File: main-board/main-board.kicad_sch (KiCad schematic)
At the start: 89 parts, among them IC13 TPS2121RUXR, J47 Barrel Jack, J6 Conn_01x03, J66 Conn_01x01_Socket, J7 Conn_Boaxial, J73 Conn_01x03, J8 USB_C_Receptacle_USB2.0_16P, J9 Conn_02x04_Odd_Even, SW1 SW_Push, SW5 SW_Push, U10 SI5351A-B-GTR, U3 TLV75801PDBV, U5 TLV75801PDBV, X1 OK322532.768KJBA4SL, Y2 NX3225GA-25.000M-STD-CRG-2

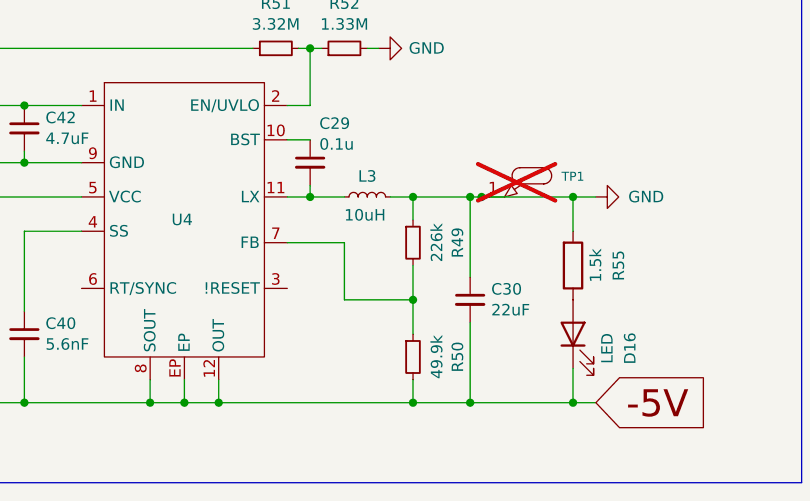
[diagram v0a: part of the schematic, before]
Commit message: pcb update
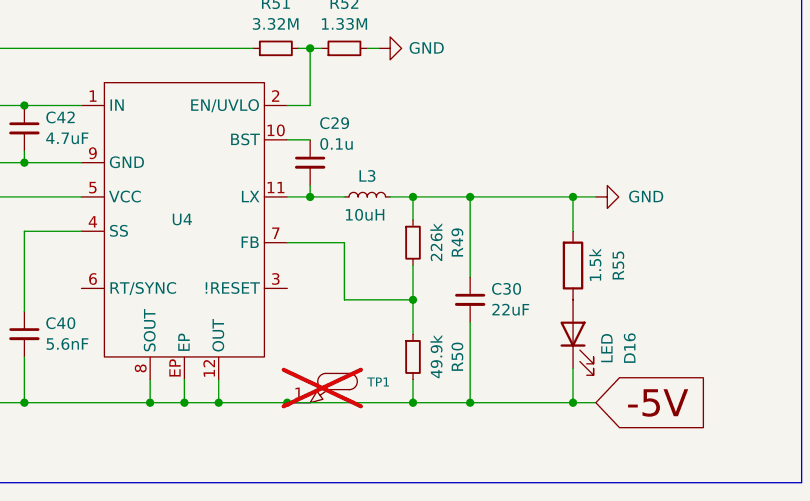
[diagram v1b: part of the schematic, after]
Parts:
- TP1, TP2, TP3, TP4, TP5, TP6: footprint Library:TP_50_28_RING -> TestPoint:TestPoint_Loop_D1.80mm_Drill1.0mm_Beaded
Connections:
- net -5V: now also TP1.1
- net GND: no longer TP1.1
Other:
- moved on the sheet: TP1
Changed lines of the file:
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@@
 	)
 	(junction
-		(at 434.34 361.95)
-		(diameter 0)
-		(color 0 0 0 0)
-	)
-	(junction
 		(at 217.17 341.63)
 		(diameter 0)
@@
 	)
 	(junction
+		(at 412.75 384.81)
+		(diameter 0)
+		(color 0 0 0 0)
+	)
+	(junction
 		(at 86.995 250.825)
 		(diameter 0)
@@
 	(wire
 		(pts
-			(xy 433.07 361.95) (xy 434.34 361.95)
-		)
-		(stroke
-			(width 0)
-			(type default)
-		)
-	)
-	(wire
-		(pts
-			(xy 434.34 361.95) (xy 444.5 361.95)
+			(xy 433.07 361.95) (xy 444.5 361.95)
 		)
 		(stroke
@@
 	(wire
 		(pts
+			(xy 412.75 384.81) (xy 426.72 384.81)
+		)
+		(stroke
+			(width 0)
+			(type default)
+		)
+	)
+	(wire
+		(pts
 			(xy 267.97 259.08) (xy 255.905 259.08)
 		)
@@
 	(wire
 		(pts
-			(xy 405.13 384.81) (xy 426.72 384.81)
+			(xy 405.13 384.81) (xy 412.75 384.81)
 		)
 		(stroke
@@
 			)
 		)
-		(property "Footprint" "Library:TP_50_28_RING"
+		(property "Footprint" "TestPoint:TestPoint_Loop_D1.80mm_Drill1.0mm_Beaded"
 			(at 281.8892 268.8082 0)
 			(effects
@@
 			)
 		)
-		(property "Footprint" "Library:TP_50_28_RING"
+		(property "Footprint" "TestPoint:TestPoint_Loop_D1.80mm_Drill1.0mm_Beaded"
 			(at 297.1292 334.4418 0)
 			(effects
@@
 			)
 		)
-		(property "Footprint" "Library:TP_50_28_RING"
+		(property "Footprint" "TestPoint:TestPoint_Loop_D1.80mm_Drill1.0mm_Beaded"
 			(at 306.0192 298.8818 0)
 			(effects
@@
 			)
 		)
-		(property "Footprint" "Library:TP_50_28_RING"
+		(property "Footprint" "TestPoint:TestPoint_Loop_D1.80mm_Drill1.0mm_Beaded"
 			(at 266.6492 241.7318 0)
 			(effects
@@
 	(symbol
 		(lib_id "Library:TP")
-		(at 434.34 361.95 0)
+		(at 412.75 384.81 0)
 		(unit 1)
 		(exclude_from_sim no)
@@
 		(fields_autoplaced yes)
 		(property "Reference" "TP1"
-			(at 443.23 359.6871 0)
+			(at 421.64 382.5471 0)
 			(effects
 				(font
@@
 		)
 		(property "Value" "~"
-			(at 443.23 361.5921 0)
+			(at 421.64 384.4521 0)
 			(effects
 				(font
@@
 			)
 		)
-		(property "Footprint" "Library:TP_50_28_RING"
-			(at 434.2892 364.9218 0)
+		(property "Footprint" "TestPoint:TestPoint_Loop_D1.80mm_Drill1.0mm_Beaded"
+			(at 412.6992 387.7818 0)
 			(effects
 				(font
@@
 		)
 		(property "Datasheet" ""
-			(at 434.34 361.95 0)
+			(at 412.75 384.81 0)
 			(effects
 				(font
@@
 		)
 		(property "Description" ""
-			(at 434.34 361.95 0)
+			(at 412.75 384.81 0)
 			(effects
 				(font
@@
 			)
 		)
-		(property "Footprint" "Library:TP_50_28_RING"
+		(property "Footprint" "TestPoint:TestPoint_Loop_D1.80mm_Drill1.0mm_Beaded"
 			(at 314.9092 241.7318 0)
 			(effects
